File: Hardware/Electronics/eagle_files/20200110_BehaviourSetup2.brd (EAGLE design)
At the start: 82.2 x 54.6 mm, 21 parts, among them Q1 IRF540, Q2 IRF540, Q3 IRF540

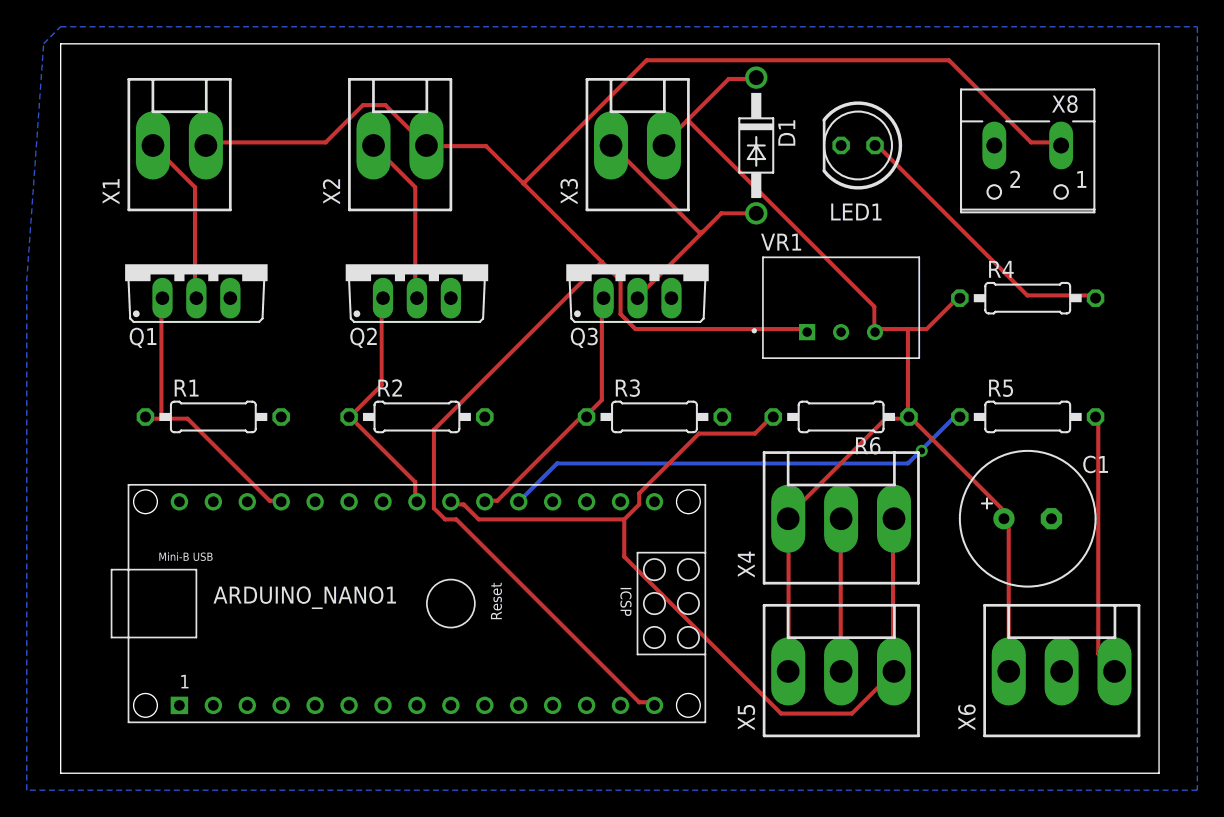
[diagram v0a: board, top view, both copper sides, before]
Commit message: Changed circuitry, rebuilt PCB
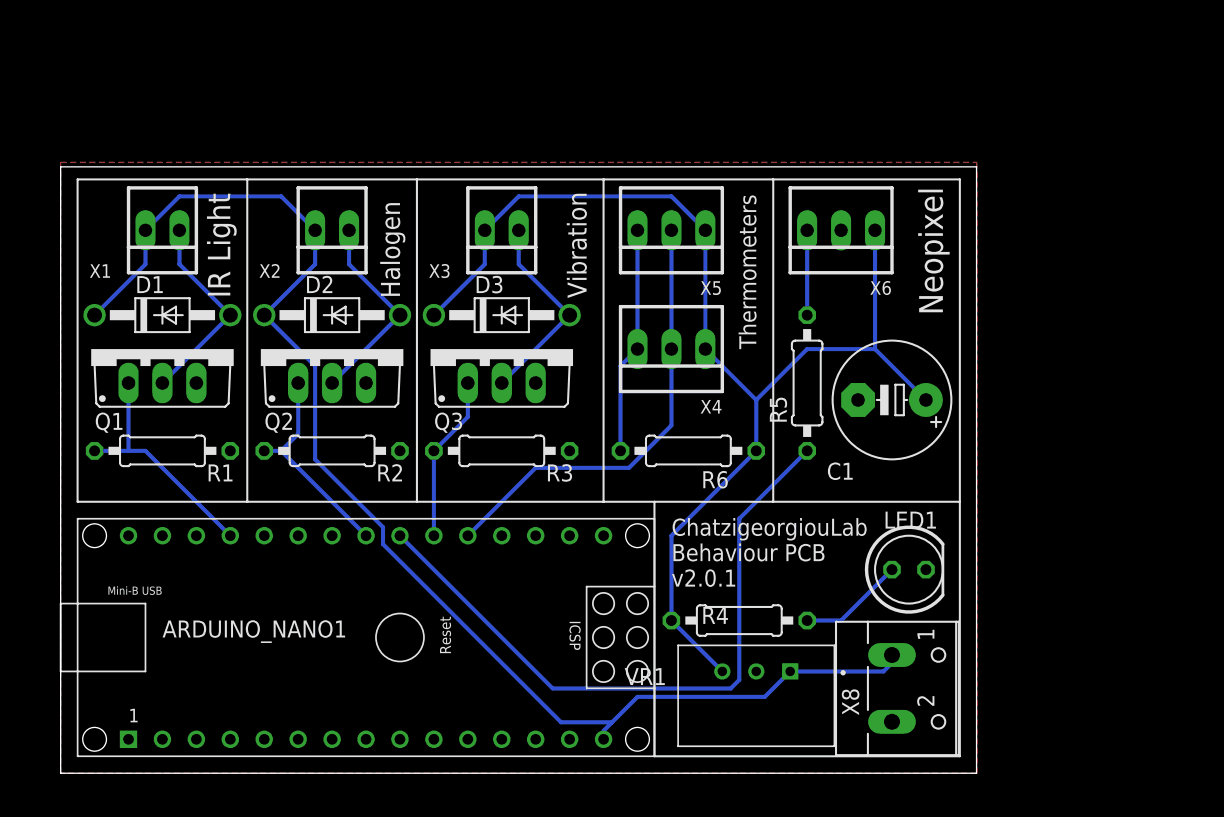
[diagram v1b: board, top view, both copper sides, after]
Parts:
- added D2, D3: 1N4004, diode:DO41-10
- C1: device rcl:E3,5-10 -> rcl:E5-8,5
- X1, X2, X3: value (none) -> 22-23-2021; device con-molex:KK-156-2 -> con-molex:22-23-2021
- X4, X5, X6: value (none) -> 22-23-2031; device con-molex:KK-156-3 -> con-molex:22-23-2031
- moved D1 46.2 mm to (7.62, 34.3), turned to 0 degrees
- moved X8 40.4 mm to (63.5, 6.35), turned to 270 degrees
- moved X6 36.9 mm to (58.4, 40.6), turned to 180 degrees
- moved X5 35.4 mm to (45.7, 40.6), turned to 180 degrees
- moved R4 32.4 mm to (50.8, 11.4)
- moved LED1 32.0 mm to (63.5, 15.2), turned to 0 degrees
- moved VR1 26.2 mm to (52.1, 7.62), turned to 180 degrees
- moved X4 18.0 mm to (45.7, 31.8), turned to 180 degrees
- moved R5 16.7 mm to (55.9, 29.2), turned to 90 degrees
- moved C1 13.5 mm to (62.2, 27.9), turned to 180 degrees
- moved Q3 12.0 mm to (33.0, 31.8)
- moved X3 12.0 mm to (33.0, 40.6), turned to 180 degrees
- moved R3 11.7 mm to (33.0, 24.1)
- moved R6 11.7 mm to (47.0, 24.1)
- moved Q2 8.98 mm to (20.3, 31.8)
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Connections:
- removed net N$2: Q1.D, X1.1
- removed net N$4: Q2.D, X2.1
- new net N$12: D2.A, Q2.D, X2.1
- new net N$13: D1.A, Q1.D, X1.1
- net +12V: now also D1.C, D2.C
- net +5V: now also D3.C; no longer D1.C
- net N$10: now also ARDUINO_NANO1.22; no longer ARDUINO_NANO1.20
- net N$6: now also D3.A; no longer D1.A
- net N$8: no longer ARDUINO_NANO1.22
- net N$9: now also ARDUINO_NANO1.20
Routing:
- net N$8: track 69.0 -> 17.0 mm
- net +12V: track 148.2 -> 99.1 mm
- net N$9: track 11.4 -> 33.3 mm
- net N$13: track 0.00 -> 15.1 mm
- net N$12: track 0.00 -> 15.1 mm
- net N$10: track 35.8 -> 49.6 mm, vias 1 -> 0
- net N$7: track 21.3 -> 7.93 mm
- net N$11: track 19.6 -> 6.35 mm
- net N$2: track 12.8 -> 0.00 mm
- net N$4: track 12.8 -> 0.00 mm
- net N$5: track 19.8 -> 12.5 mm
- net N$6: track 21.1 -> 15.1 mm
- net N$1: track 21.9 -> 17.9 mm
- net N$3: track 18.5 -> 15.9 mm
- net +5V: track 90.7 -> 90.1 mm
- added copper zone on layer 1, net GND
- removed copper zone on layer 16, net GND
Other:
- board size 82.2 x 54.6 mm -> 68.6 x 45.4 mm
- board text added: "ChatzigeorgiouLab Behaviour PCB v2.0.1"
- board text added: "Halogen"
- board text added: "IR Light"
- board text added: "Neopixel"
- board text added: "Thermometers"
- board text added: "Vibration"
